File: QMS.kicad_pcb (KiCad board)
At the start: 2 copper layers, 58.4 x 63.5 mm, 12 parts, among them J4 Conn_02x08_Top_Bottom, J6 Screw_Terminal_01x02, J7 PINHD_1x5_Male, J8 PINHD_1x5_Male, U4 ESP-12E, U5 AMS1117-3.3

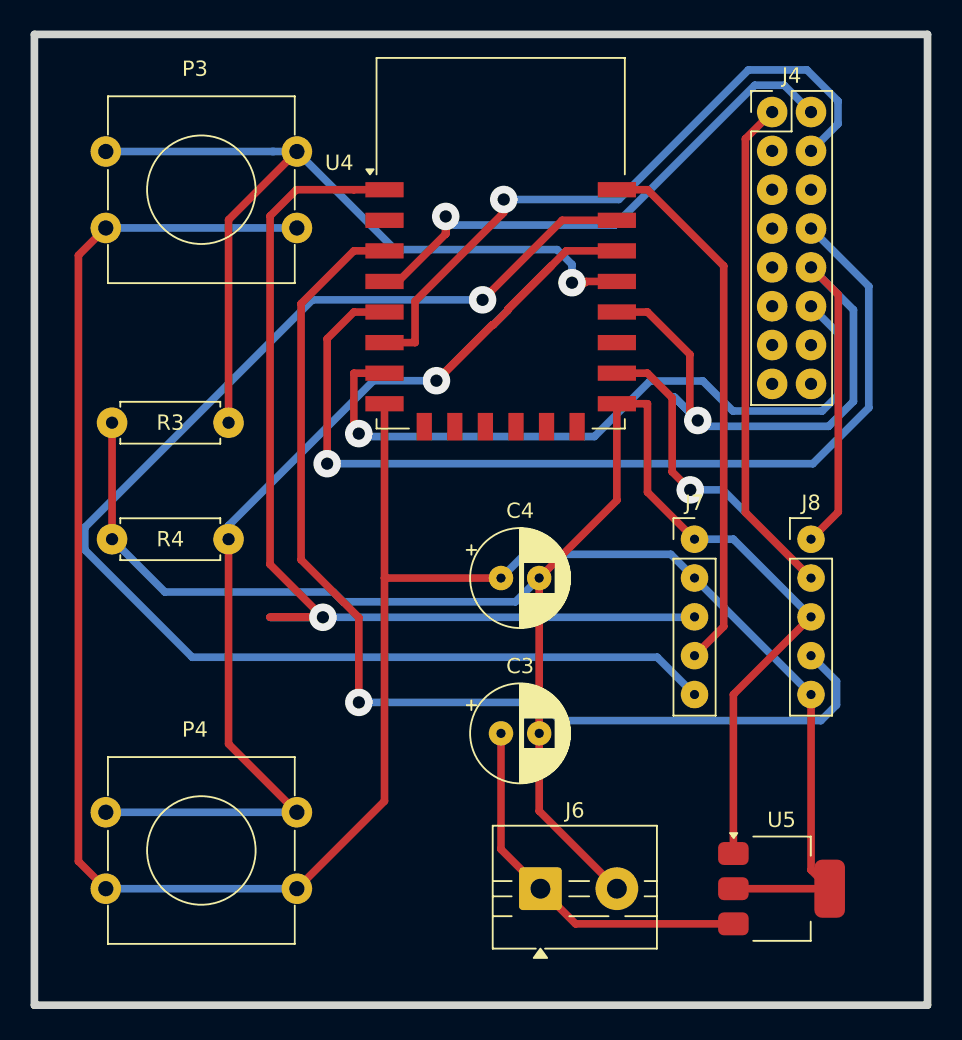
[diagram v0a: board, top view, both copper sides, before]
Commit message: some small fixes
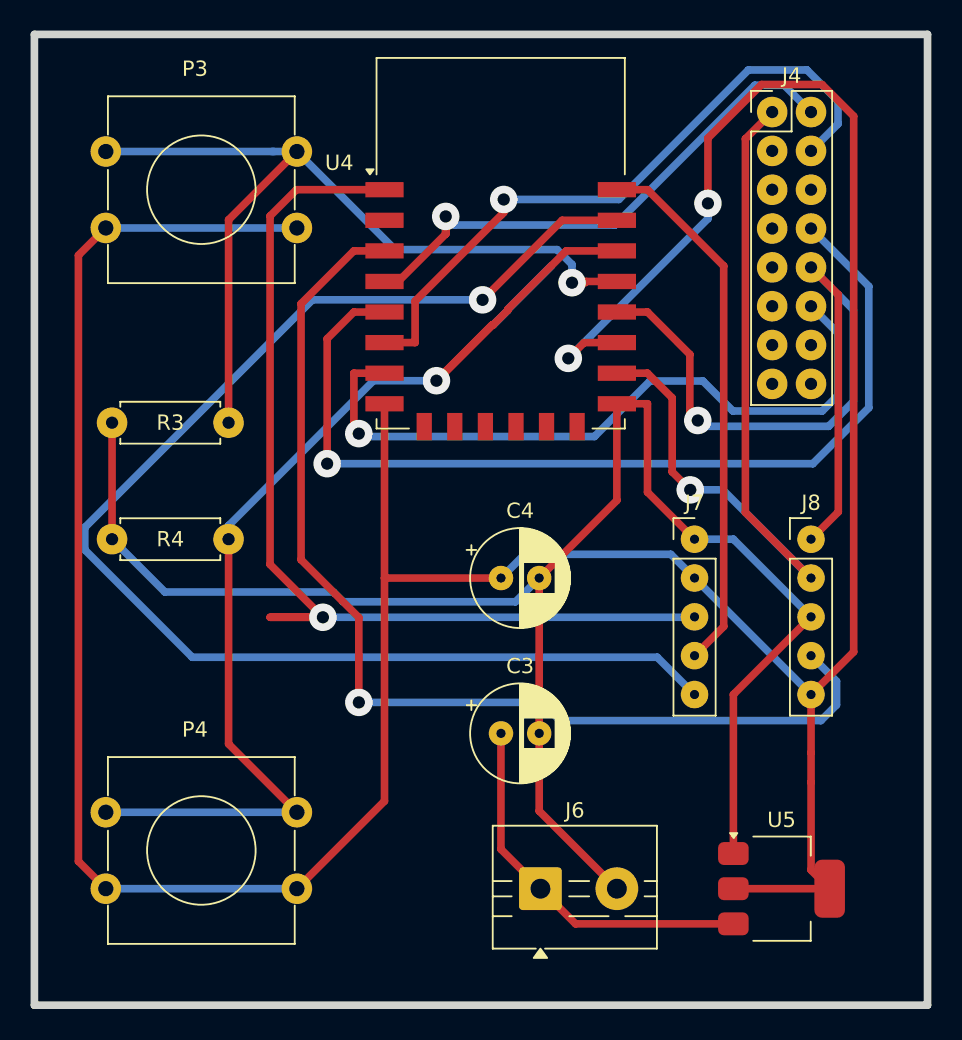
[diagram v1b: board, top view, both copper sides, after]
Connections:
- U4 pad 17: /GPIO2 -> /VCC
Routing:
- net /VCC: track 155.6 -> 231.2 mm, vias 0 -> 2
- net /GPIO5: track 104.2 -> 96.1 mm
- net /RST: track 74.0 -> 67.1 mm
- net /GPIO0: track 56.5 -> 52.1 mm
